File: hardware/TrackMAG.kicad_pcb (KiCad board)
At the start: 4 copper layers, 36 x 36 mm, 54 parts, among them J1 USB_C_Socket_USB2.0, J2 Conn_Debug, SW1 SW_RESET, SW2 SW_BOOT, U1 LSM6DS3TR-C, U2 USBLC6-2P6, U3 STM32F103C8T6, U4 LIS2MDL, U5 AMS1117-3.3, Y1 16MHz

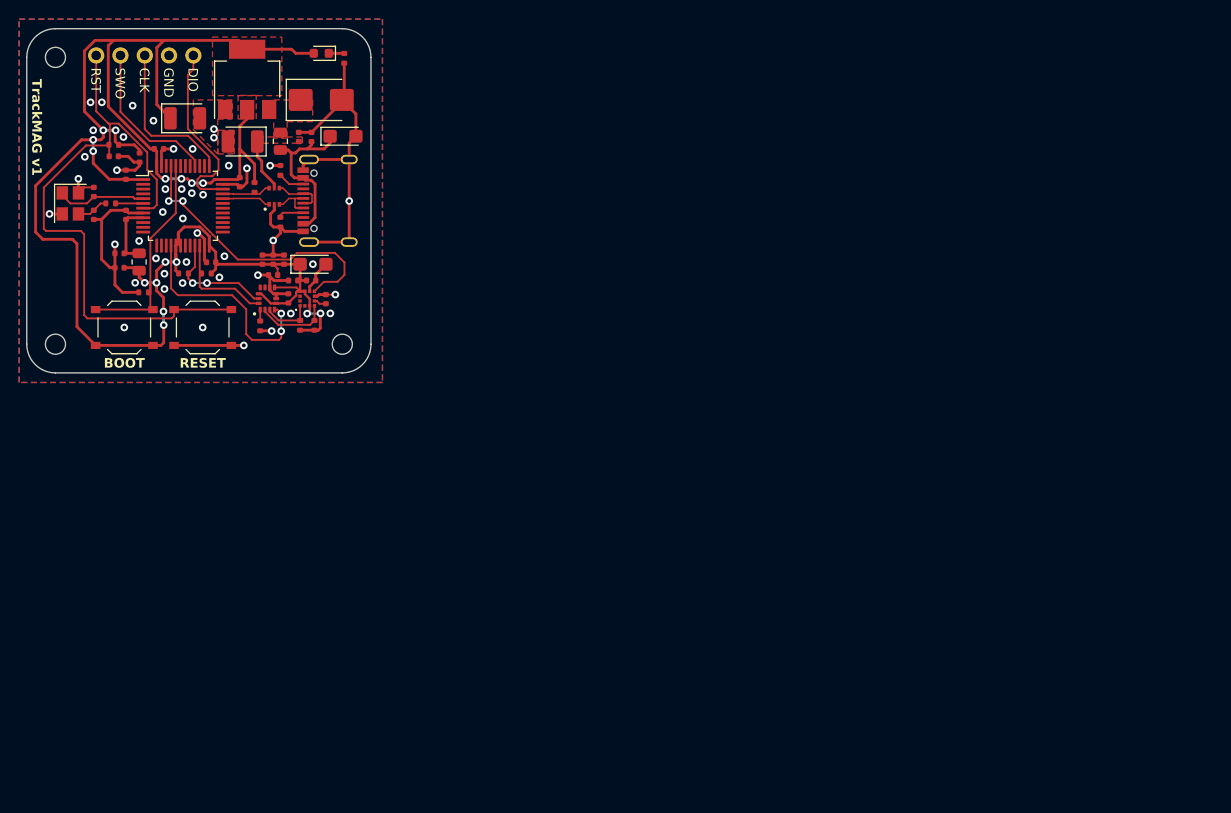
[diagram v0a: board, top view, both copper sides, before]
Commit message: Center PCB
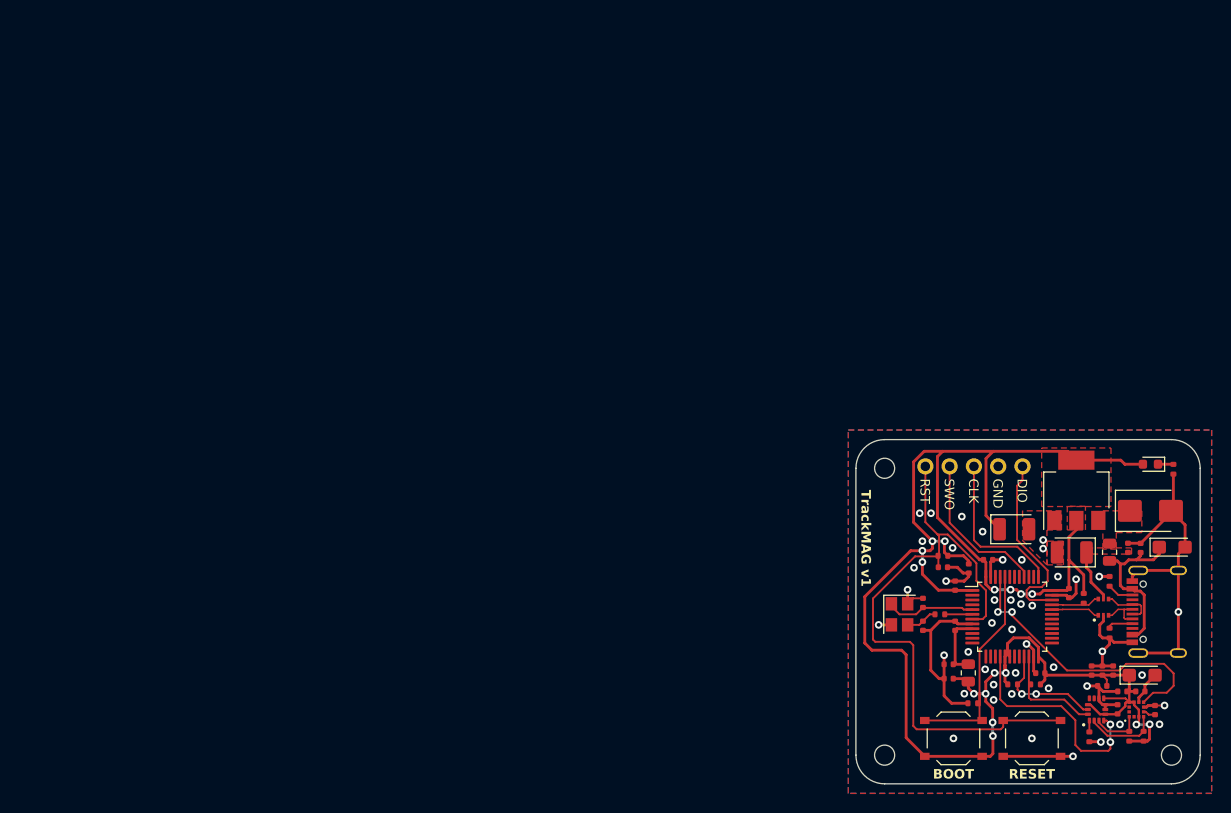
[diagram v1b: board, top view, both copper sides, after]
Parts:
- moved C21 96.8 mm to (131.5, 92.1)
- moved C24 96.8 mm to (147.1, 86.8)
- moved U5 96.8 mm to (147.6, 80.3)
- moved C10 96.8 mm to (134.9, 90.2)
- moved C12 96.8 mm to (146.8, 91.0)
- moved C13 96.8 mm to (143.8, 99.4)
- moved C14 96.8 mm to (134.9, 94.5)
- moved C19 96.8 mm to (154.3, 86.3)
- moved C23 96.8 mm to (155.8, 103.3)
- moved C25 96.8 mm to (141.1, 84.3)
- moved C6 96.8 mm to (154.3, 101.3)
- moved C8 96.8 mm to (154.5, 99.6)
- moved FB1 96.8 mm to (136.3, 99.4)
- moved FB2 96.8 mm to (151.0, 86.8)
- moved H3 96.8 mm to (157.5, 108.0)
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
